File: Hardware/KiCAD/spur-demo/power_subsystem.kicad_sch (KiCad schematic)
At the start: 35 parts, among them IC1 BQ24193RGER, IC3 ISL91127IRNZ-T7A, J5 Conn_01x02, Q1 ZXMN2A01F

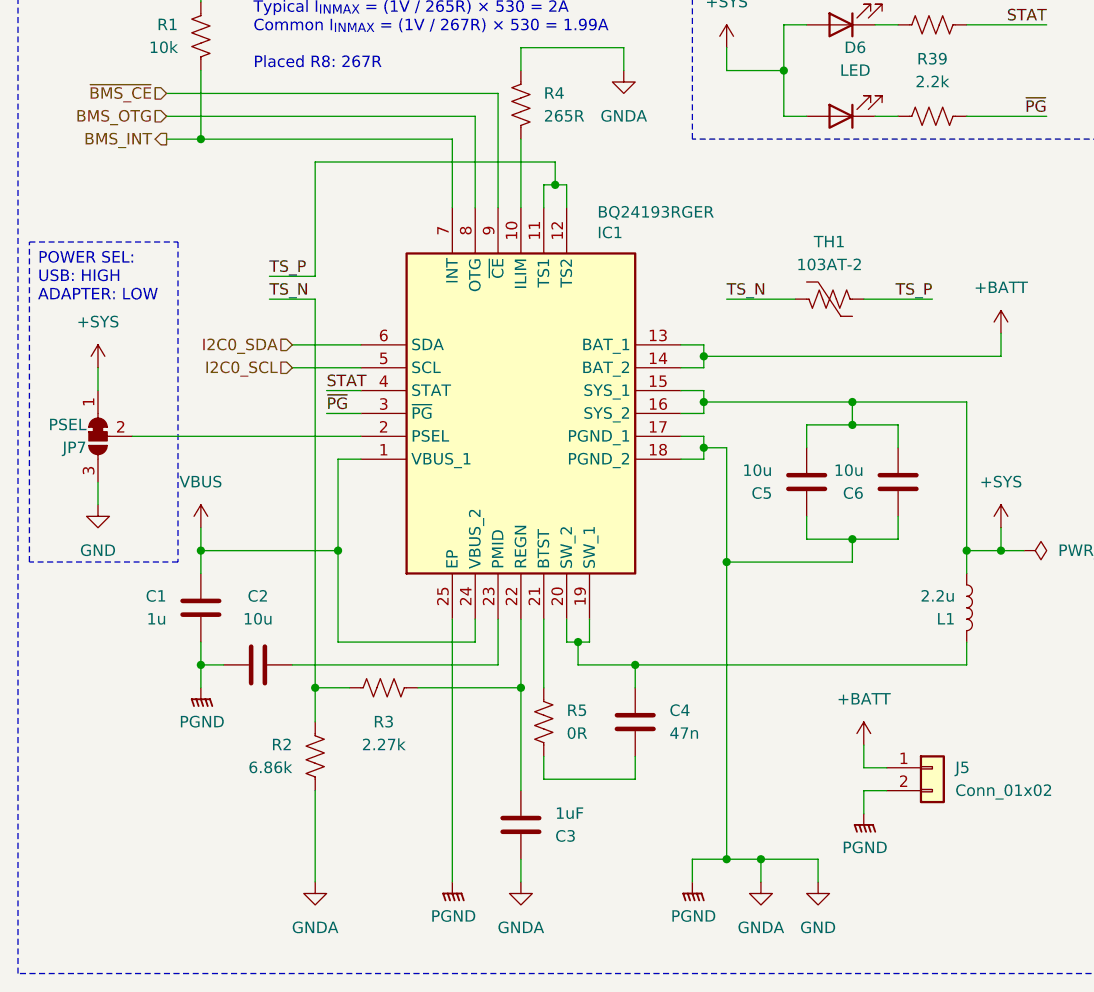
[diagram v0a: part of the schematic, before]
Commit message: fix: correct NTC thermistor resistor network
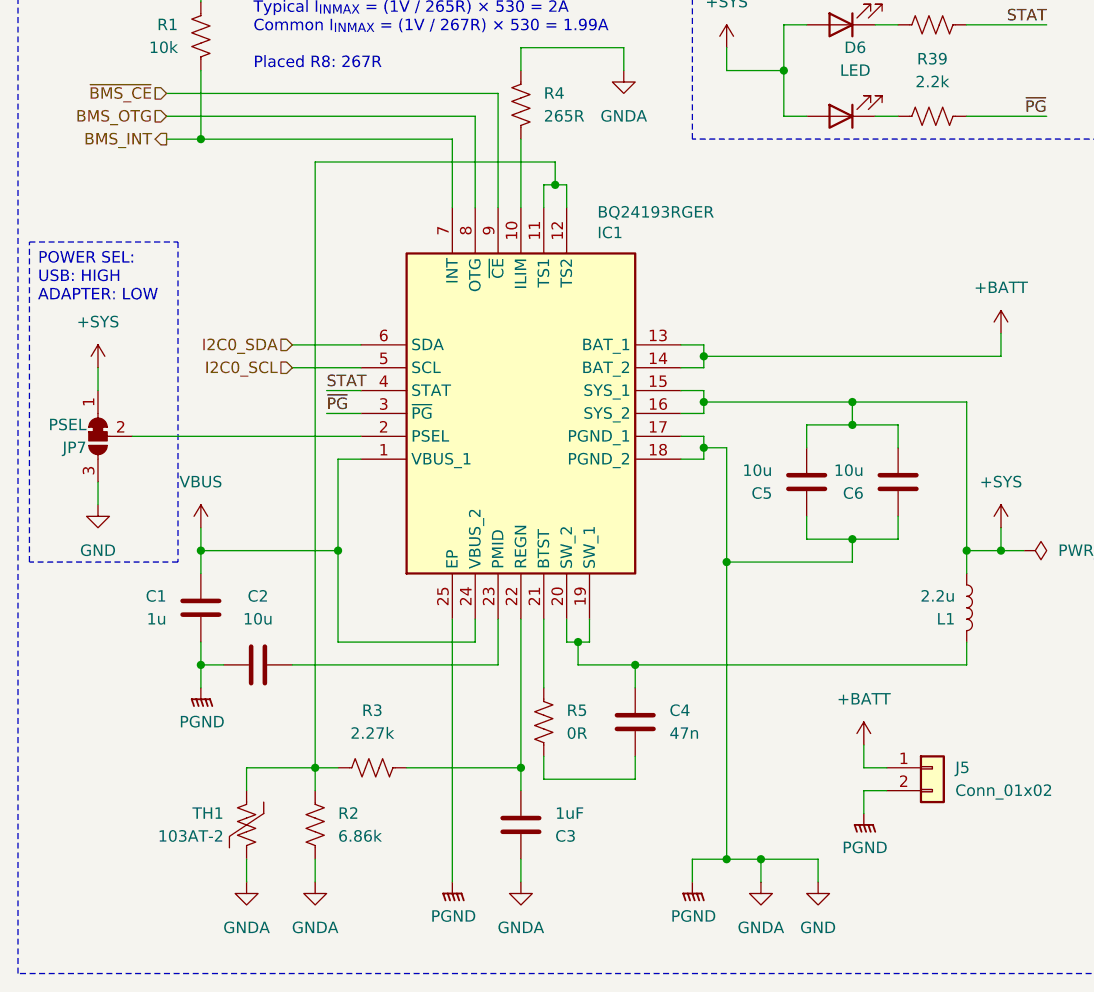
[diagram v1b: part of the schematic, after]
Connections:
- net TS_P is gone; now on an unnamed net: IC1.11 (TS1), IC1.12 (TS2), TH1.2
- net GND: now also TH1.1
- net TS_N: no longer names the net of R2.1, R3.2
- net TS_N: no longer TH1.1
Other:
- moved on the sheet: R2, R3, TH1
